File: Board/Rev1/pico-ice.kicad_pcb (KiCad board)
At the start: 4 copper layers, 22.9 x 61 mm, 97 parts, among them J1 USB_C_Receptacle_USB2.0, J2 Conn_02x20_Odd_Even, J3 Conn_02x20_Odd_Even, J4 PB_SEL, Q1 2N7002, SW1 PTS820 J25K SMTR LFS, SW2 PTS820 J25K SMTR LFS, U1 CL9293A12L5M, U2 W25Q32JVSSIQ, U3 RP2040, U4 CL9293A33L5M, U5 APS6404L-3SQN-SN, U6 ICE40UP5K-SG48ITR, U8 W25Q32JVSSIQ, Y1 12 MHz

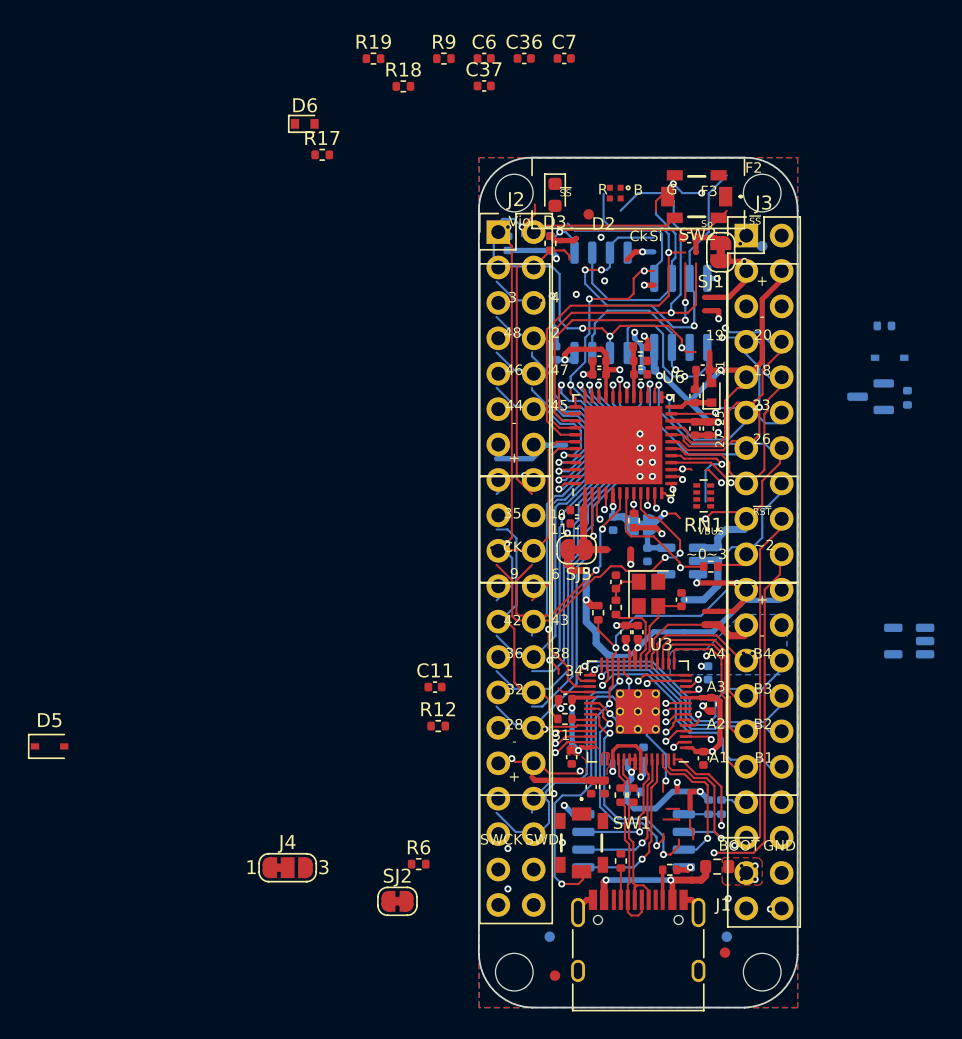
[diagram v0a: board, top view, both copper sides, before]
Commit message: Update pico-ice.kicad_pcb
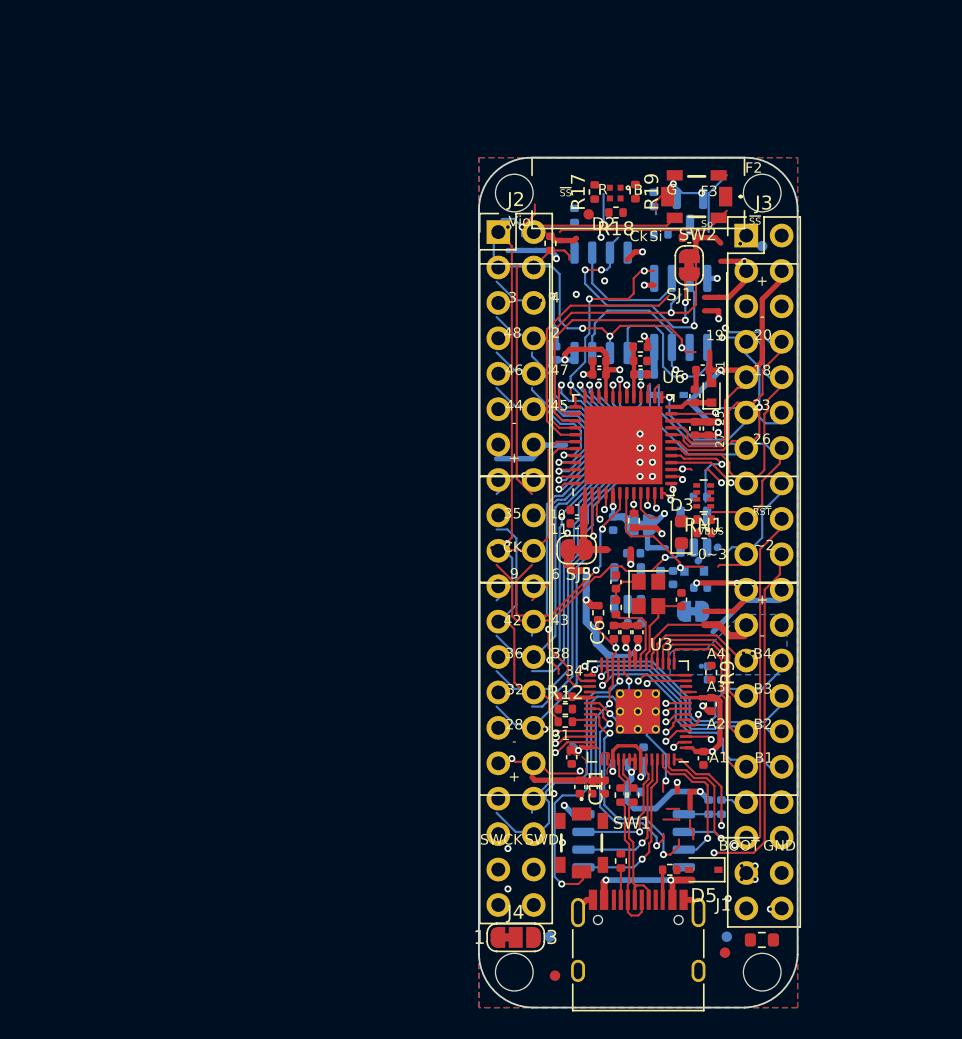
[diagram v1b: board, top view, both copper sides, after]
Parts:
- C36, C37, C7, D6, R6, SJ2: moved to B.Cu
- R14: moved to F.Cu
- moved R9 48.0 mm to (77.6, 110.6), turned to -90 degrees
- moved D5 47.7 mm to (77.1, 124.7), turned to 180 degrees
- moved D6 42.5 mm to (76.4, 103.3), turned to 180 degrees
- moved C6 42.2 mm to (70.6, 107.7), turned to 90 degrees
- moved C7 40.8 mm to (72.1, 107.1), turned to 180 degrees
- moved C36 38.7 mm to (74.9, 103.8), turned to -90 degrees
- moved C37 35.2 mm to (72.1, 102.0), turned to 180 degrees
- moved SJ2 29.7 mm to (76.3, 106.2), turned to 180 degrees
- moved R6 26.9 mm to (74.0, 103.8), turned to 90 degrees
- moved D3 25.8 mm to (75.5, 100.5), turned to 90 degrees
- moved R14 25.1 mm to (77.1, 100.6), turned to 0 degrees
- moved R13 23.1 mm to (73.5, 76.7), turned to -90 degrees
- moved R19 21.1 mm to (72.2, 76.1), turned to -90 degrees
- moved U1 20.5 mm to (71.6, 104.5), turned to 90 degrees
- moved R17 19.7 mm to (69.3, 76.1), turned to 90 degrees
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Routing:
- net +3V3: track 214.1 -> 171.5 mm, vias 26 -> 21
- net +1V2: track 0.00 -> 19.3 mm, vias 0 -> 2
- net /ICE_SSN: track 15.6 -> 1.26 mm, vias 1 -> 0
- net /~{ICE_RST}: track 479.0 -> 466.7 mm
- net /LED_B: track 35.5 -> 24.0 mm
- net /LED_R: track 31.4 -> 21.2 mm, vias 1 -> 0
- net /SRAM_SS: track 52.7 -> 43.2 mm
- net GND: track 470.3 -> 463.1 mm, vias 52 -> 43
- net /ICE_FLASH_IO2: track 44.6 -> 38.2 mm
- net /ICE_6: track 66.8 -> 61.0 mm, vias 5 -> 4
- net /ICE_9: track 12.9 -> 15.5 mm
- net /PICO_PMOD_B2: track 2.37 -> 0.00 mm
- net VDC: track 10.9 -> 9.11 mm
- net /+3V3_STDBY: track 0.00 -> 1.66 mm
- net /ICE_27: track 0.00 -> 1.02 mm
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- removed copper zone on F.Cu, net VBUS
